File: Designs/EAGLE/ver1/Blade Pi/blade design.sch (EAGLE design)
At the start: 35 parts

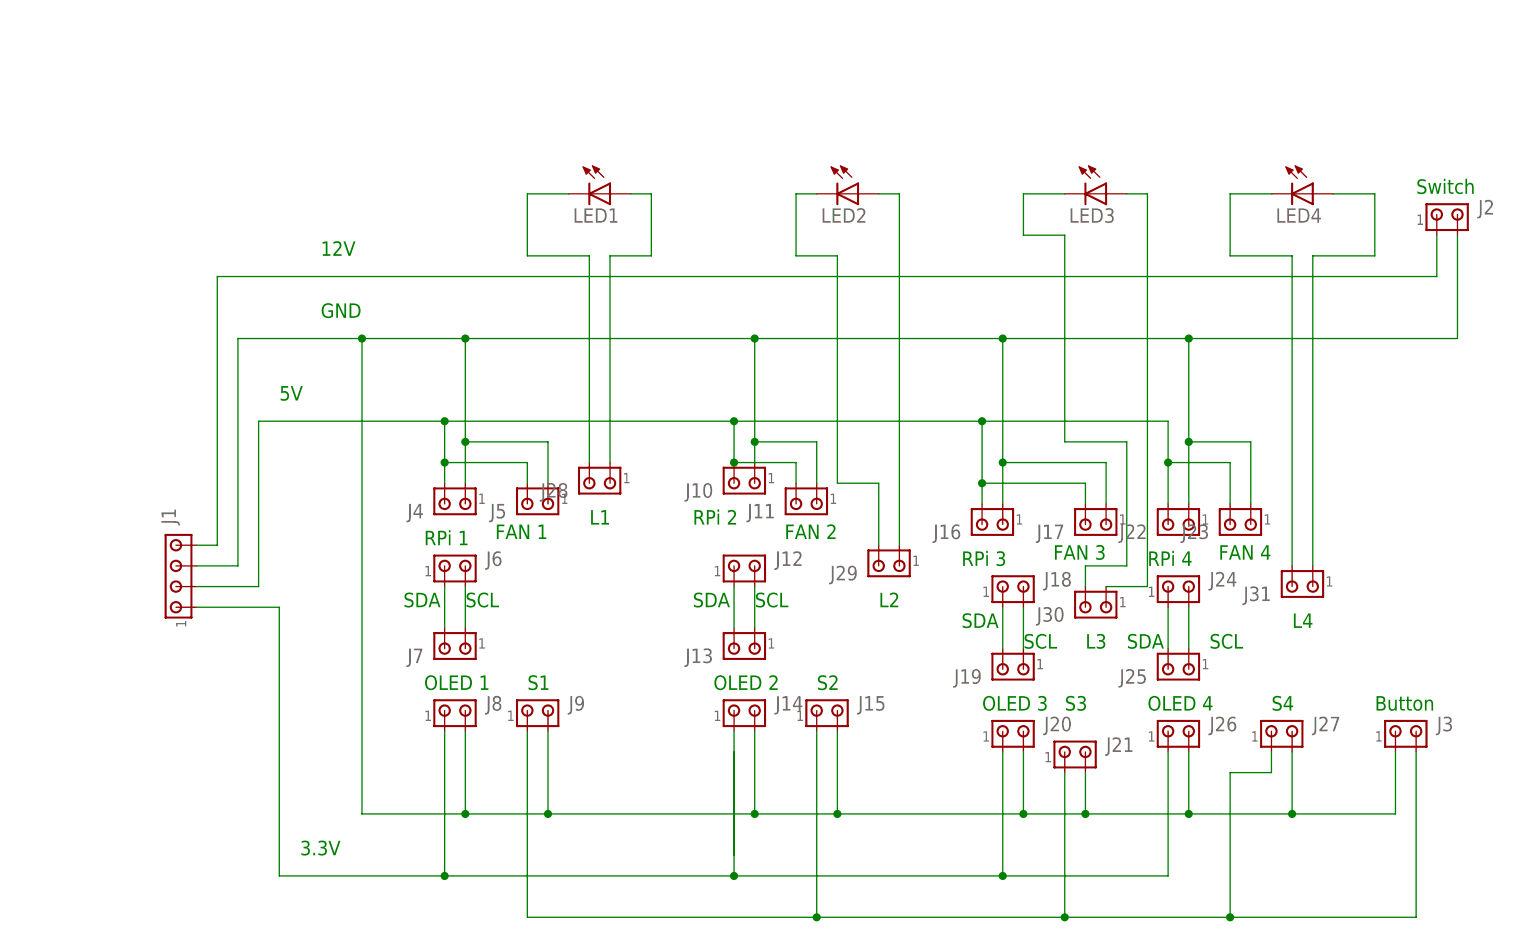
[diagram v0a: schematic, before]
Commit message: board design complete
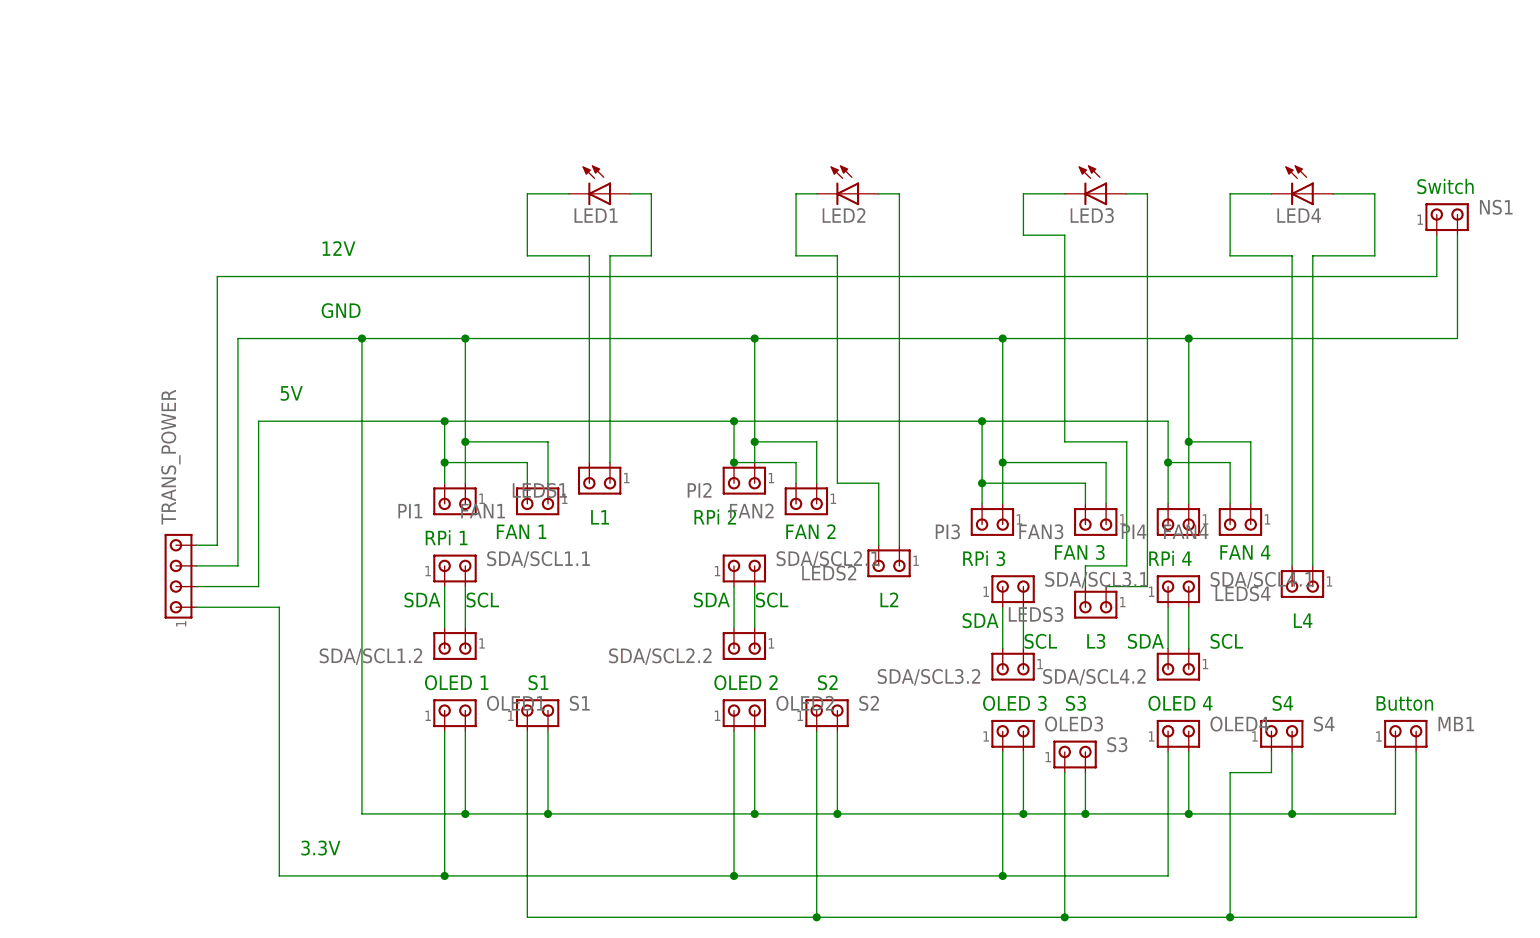
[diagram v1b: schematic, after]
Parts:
- renumbered J1 to TRANS_POWER, J10 to PI2, J11 to FAN2, J12 to SDA/SCL2.1, J13 to SDA/SCL2.2, J14 to OLED2, J15 to S2, J16 to PI3, J17 to FAN3, J18 to SDA/SCL3.1, J19 to SDA/SCL3.2, J2 to NS1, J20 to OLED3, J21 to S3, J22 to PI4, J23 to FAN4, J24 to SDA/SCL4.1, J25 to SDA/SCL4.2, J26 to OLED4, J27 to S4, J28 to LEDS1, J29 to LEDS2, J3 to MB1, J30 to LEDS3, J31 to LEDS4, J4 to PI1, J5 to FAN1, J6 to SDA/SCL1.1, J7 to SDA/SCL1.2, J8 to OLED1, J9 to S1
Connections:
- net N$1 renamed 12V
- net N$3 renamed 5V
- removed net N$13: MB1.2, S1.1, S3.1, S4.1
- removed net N$4: FAN1.1, FAN2.1, FAN3.1, FAN4.1, MB1.1, NS1.2, OLED1.2, OLED3.2, OLED4.2, PI1.1, PI2.1, PI3.1, PI4.1, S1.2, S3.2, S4.2, TRANS_POWER.3
- removed net N$5: OLED1.1, OLED3.1, OLED4.1, TRANS_POWER.1
- new net 3.3V: OLED1.1, OLED2.1, OLED3.1, OLED4.1, TRANS_POWER.1
- new net GND: FAN1.1, FAN2.1, FAN3.1, FAN4.1, MB1.1, NS1.2, OLED1.2, OLED2.2, OLED3.2, OLED4.2, PI1.1, PI2.1, PI3.1, PI4.1, S1.2, S2.2, S3.2, S4.2, TRANS_POWER.3
- new net PS: MB1.2, S1.1, S2.1, S3.1, S4.1

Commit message: First design complete
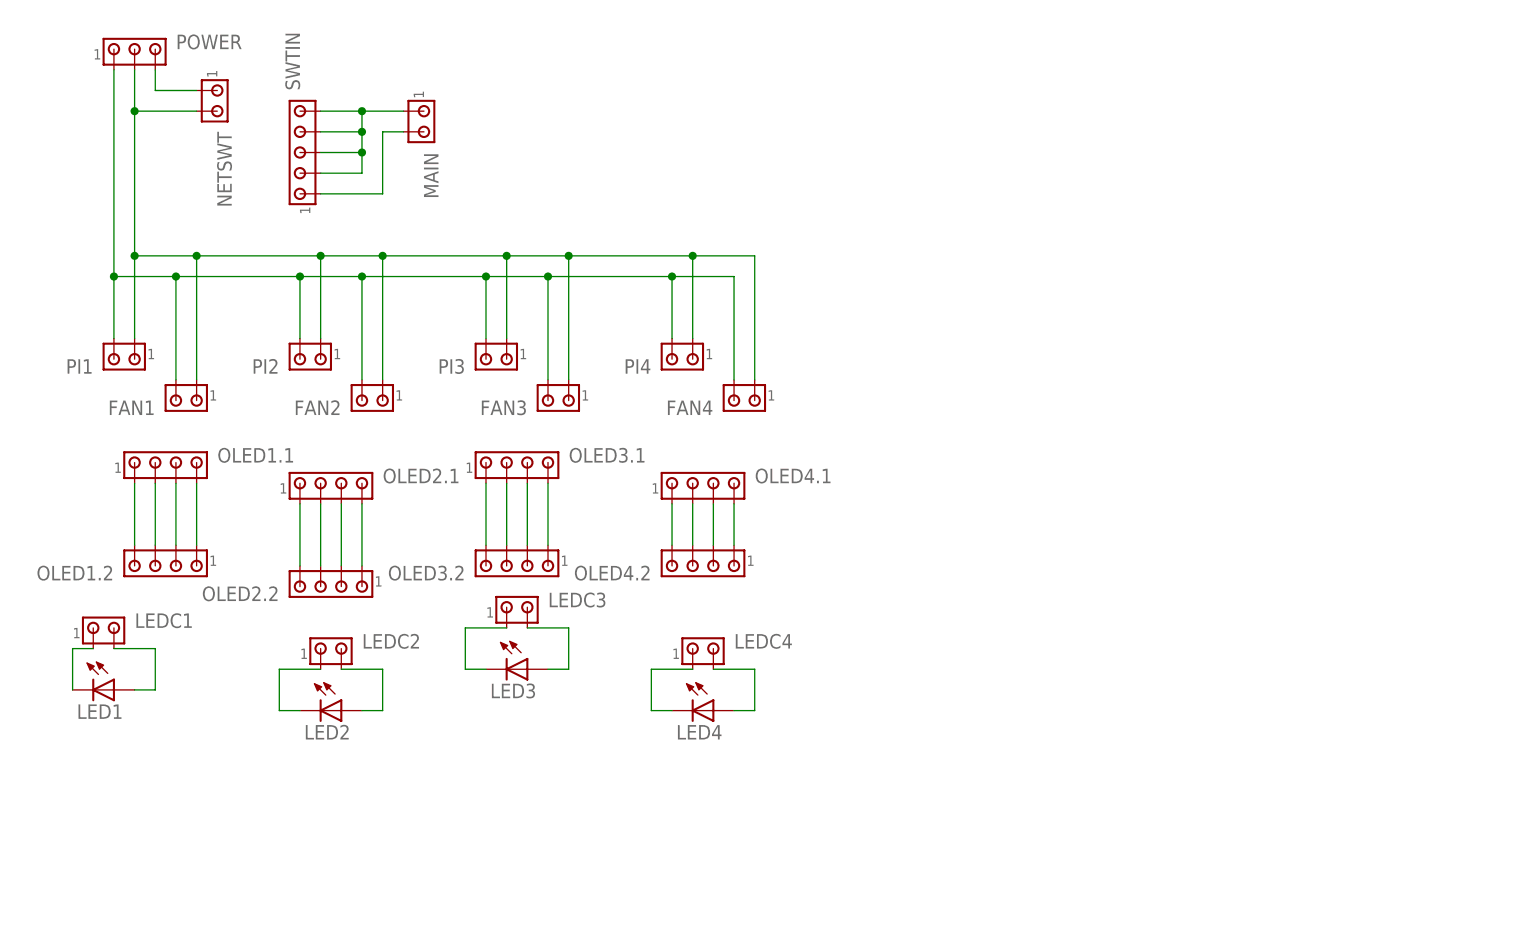
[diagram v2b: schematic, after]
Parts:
- removed LEDS1, LEDS2, LEDS3, LEDS4, OLED1, OLED2, OLED3, OLED4, S1, S2, S3, S4, SDA/SCL1.1, SDA/SCL1.2, SDA/SCL2.1, SDA/SCL2.2, SDA/SCL3.1, SDA/SCL3.2, SDA/SCL4.1, SDA/SCL4.2: (no value), con-amp:MTA02-156
- removed MB1, NS1: (no value), con-amp:MTA02-100
- removed TRANS_POWER: (no value), con-amp:MTA04-100
- added LEDC1, LEDC2, LEDC3, LEDC4, MAIN, NETSWT: (no value), con-amp:MTA02-156
- added OLED1.1, OLED1.2, OLED2.1, OLED2.2, OLED3.1, OLED3.2, OLED4.1, OLED4.2: (no value), con-amp:MTA04-156
- added POWER: (no value), con-amp:MTA03-156
- added SWTIN: (no value), con-amp:MTA05-156
- LED1, LED2, LED3, LED4: device eagle-ltspice:LED_E -> eagle-ltspice:LED_ELD260
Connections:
- removed net N$10: SDA/SCL3.1.2, SDA/SCL3.2.1
- removed net N$11: SDA/SCL4.1.1, SDA/SCL4.2.2
- removed net N$12: SDA/SCL4.1.2, SDA/SCL4.2.1
- removed net N$14: LED1.C, LEDS1.2
- removed net N$15: LED1.A, LEDS1.1
- removed net N$16: LED2.C, LEDS2.2
- removed net N$17: LED2.A, LEDS2.1
- removed net N$18: LED3.C, LEDS3.2
- removed net N$20: LED4.C, LEDS4.2
- removed net N$21: LED4.A, LEDS4.1
- removed net N$22: LED3.A, LEDS3.1
- removed net N$9: SDA/SCL3.1.1, SDA/SCL3.2.2
- removed net PS: MB1.2, S1.1, S2.1, S3.1, S4.1
- new net GND1: OLED1.1.1, OLED1.2.4
- new net GND2: OLED2.1.1, OLED2.2.4
- new net GND3: OLED3.1.1, OLED3.2.4
- new net GND4: OLED4.1.1, OLED4.2.4
- new net N$1: LED1.C, LEDC1.1
- new net N$3: LED2.C, LEDC2.1
- new net N$4: LED2.A, LEDC2.2
- new net N$5: LED3.C, LEDC3.1
- new net SCL1: OLED1.1.3, OLED1.2.2
- new net SCL2: OLED2.1.3, OLED2.2.2
- new net SCL3: OLED3.1.3, OLED3.2.2
- new net SCL4: OLED4.1.3, OLED4.2.2
- new net SDA1: OLED1.1.4, OLED1.2.1
- new net SDA2: OLED2.1.4, OLED2.2.1
- new net SDA3: OLED3.1.4, OLED3.2.1
- new net SDA4: OLED4.1.4, OLED4.2.1
- new net SWTCH: MAIN.1, SWTIN.2, SWTIN.3, SWTIN.4, SWTIN.5
- new net VCC1: OLED1.1.2, OLED1.2.3
- new net VCC2: OLED2.1.2, OLED2.2.3
- new net VCC3: OLED3.1.2, OLED3.2.3
- new net VCC4: OLED4.1.2, OLED4.2.3
- net 12V: now also NETSWT.1, POWER.3; no longer NS1.1, TRANS_POWER.4
- net 3.3V: now also MAIN.2, SWTIN.1; no longer OLED1.1, OLED2.1, OLED3.1, OLED4.1, TRANS_POWER.1
- net 5V: now also POWER.1; no longer TRANS_POWER.2
- net GND: now also NETSWT.2, POWER.2; no longer MB1.1, NS1.2, OLED1.2, OLED2.2, OLED3.2, OLED4.2, S1.2, S2.2, S3.2, S4.2, TRANS_POWER.3
- net N$2: now also LED1.A, LEDC1.2; no longer SDA/SCL1.1.1, SDA/SCL1.2.2
- net N$6: now also LED3.A, LEDC3.2; no longer SDA/SCL1.1.2, SDA/SCL1.2.1
- net N$7: now also LED4.C, LEDC4.1; no longer SDA/SCL2.1.1, SDA/SCL2.2.2
- net N$8: now also LED4.A, LEDC4.2; no longer SDA/SCL2.1.2, SDA/SCL2.2.1
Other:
- note removed: "12V"
- note removed: "3.3V"
- note removed: "5V"
- note removed: "Button"
- note removed: "FAN 1"
- note removed: "FAN 2"
- note removed: "FAN 3"
- note removed: "FAN 4"
- note removed: "GND"
- note removed: "L1"
- note removed: "L2"
- note removed: "L3"
- note removed: "L4"
- note removed: "OLED 1"
- note removed: "OLED 2"
- note removed: "OLED 3"
- note removed: "OLED 4"
- note removed: "RPi 1"
- note removed: "RPi 2"
- note removed: "RPi 3"
- note removed: "RPi 4"
- note removed: "S1"
- note removed: "S2"
- note removed: "S3"
- note removed: "S4"
- note removed: "SCL"
- note removed: "SDA"
- note removed: "Switch"
- moved on the sheet: FAN1, FAN2, FAN3, FAN4, LED1, LED2, LED3, LED4, PI1, PI2, PI3, PI4
